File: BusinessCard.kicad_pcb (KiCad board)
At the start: 2 copper layers, 85.6 x 54 mm, 29 parts, among them U1 NT3H2111W0FHKH

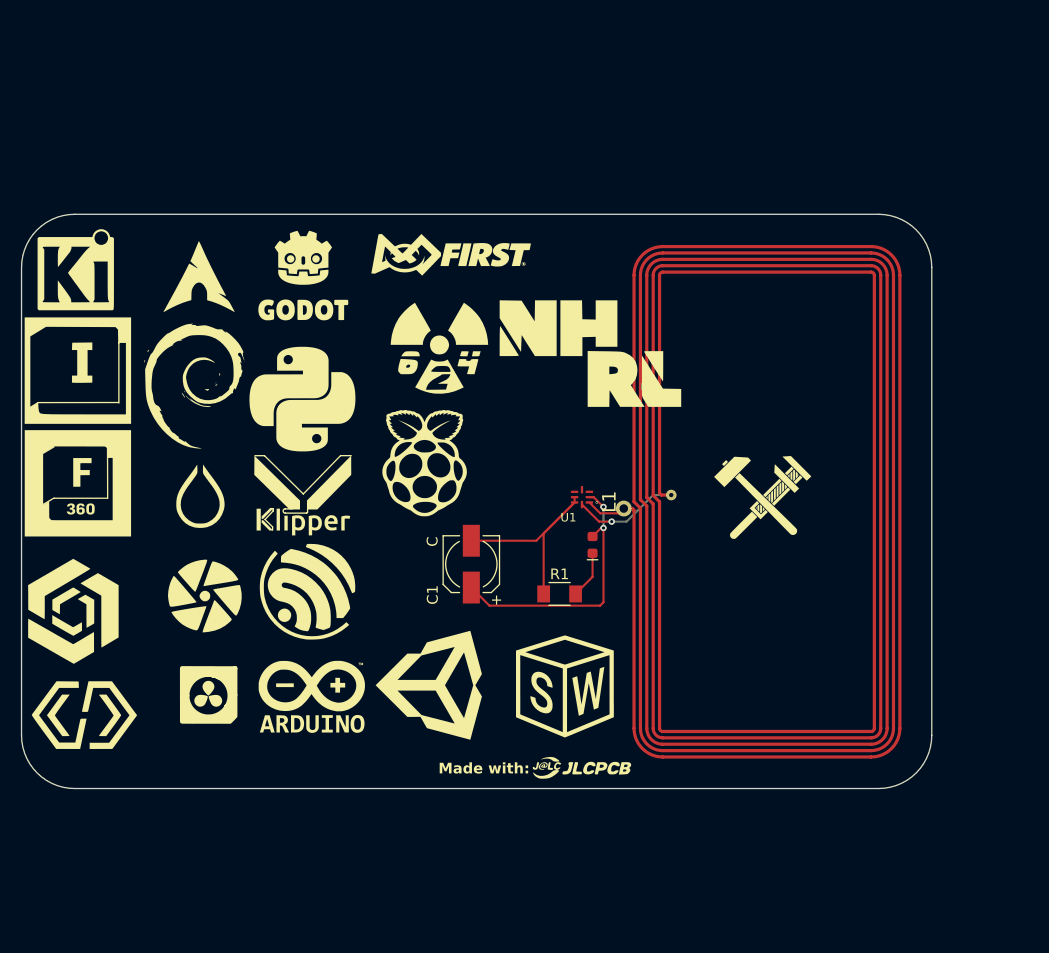
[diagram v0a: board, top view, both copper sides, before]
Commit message: Made a few design changes, started the intro
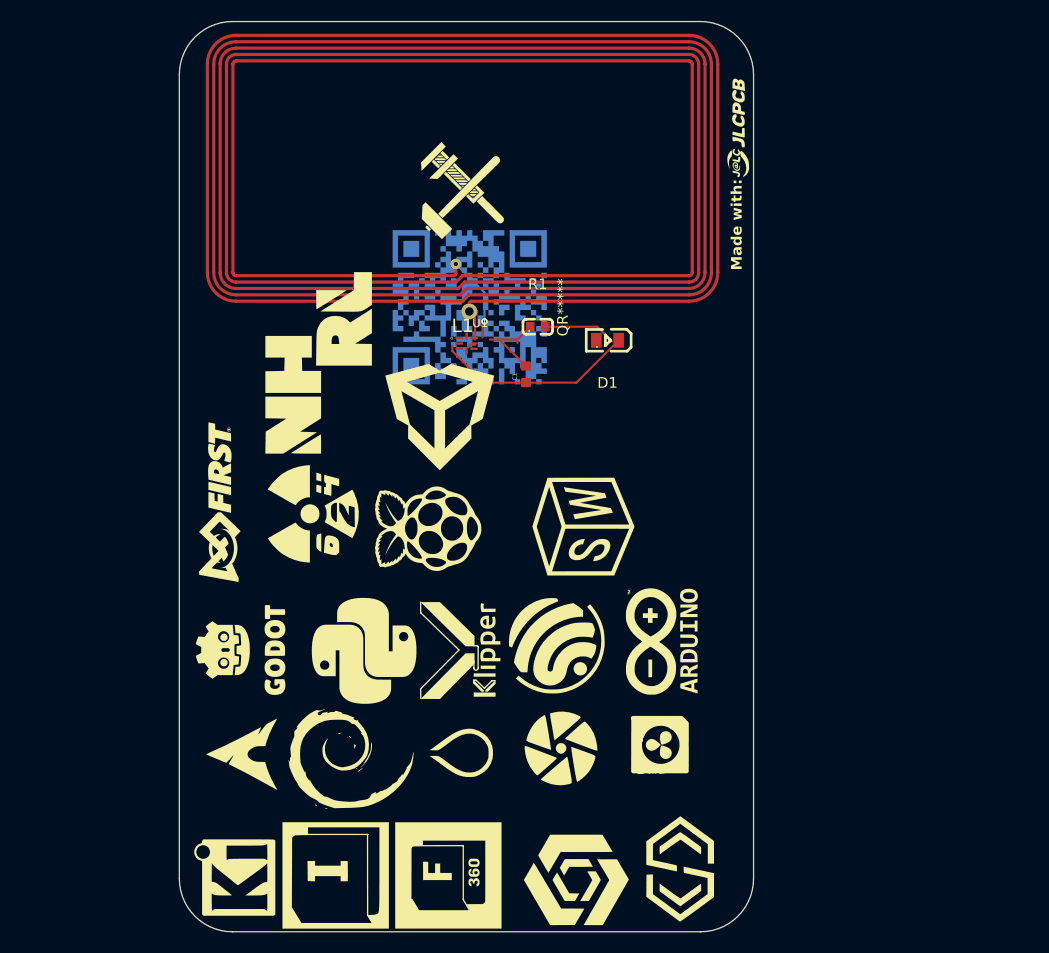
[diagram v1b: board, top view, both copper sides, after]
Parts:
- added QR*****: https://github.com/JudasLilith, nfc:https___github.com_JudasLilith, B.Cu at (116.0, 74.8)
- C1: footprint PCM_4ms_Capacitor:CP_Elec_5x5.3 -> nfc:CAPC1608X90N
- D1: footprint PCM_SparkFun-LED:LED_0603_1608Metric -> nfc:LED0805-R-RD
- R1: footprint PCM_fab:R_1206 -> nfc:C0603
- moved G*** 62.0 mm to (141.3, 57.9), turned to 90 degrees
- moved G*** 59.0 mm to (94.0, 128.4), turned to 90 degrees
- moved G*** 57.8 mm to (135.7, 127.6), turned to 90 degrees
- moved G*** 53.5 mm to (126.1, 128.5), turned to 90 degrees
- moved G*** 53.3 mm to (103.4, 128.2), turned to 90 degrees
- moved G*** 50.7 mm to (114.0, 128.2), turned to 90 degrees
- moved G*** 44.3 mm to (95.4, 116.8), turned to 90 degrees
- moved L1 42.5 mm to (115.4, 61.7), turned to 180 degrees
- moved G*** 40.4 mm to (115.4, 63.8), turned to 90 degrees
- moved G*** 40.0 mm to (133.9, 113.4), turned to 90 degrees
- moved G*** 38.0 mm to (104.8, 117.2), turned to 90 degrees
- moved G*** 34.9 mm to (95.2, 107.0), turned to 90 degrees
- moved G*** 34.4 mm to (115.2, 116.7), turned to 90 degrees
- moved G*** 33.4 mm to (134.1, 106.2), turned to 90 degrees
- moved G*** 31.9 mm to (92.5, 93.1), turned to 90 degrees
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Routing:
- net Net-(C1--): track 21.5 -> 7.87 mm
- net Net-(C1-+): track 25.3 -> 19.7 mm, vias 2 -> 0
- net Net-(D1-K): track 4.49 -> 6.88 mm
- net Net-(U1-LB): track 10.1 -> 8.21 mm
- net Net-(U1-LA): track 3.66 -> 3.05 mm
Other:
- board size 85.6 x 54 mm -> 54 x 85.6 mm
- board text added: "+1(346)-287-4367"
- board text added: "-Beginner GameDev & WebDev"
- board text added: "-FRC,NTHS,TSA & Hack Club"
- board text added: "-Hobby CAD student"
- board text added: "-Hobby Mill and CNC machinist"
- board text added: "-PCB designer"
- board text added: "-Supreme™ Archlinux user"
- board text added: "He/him"
- board text added: "Judaslilith.com"
- board text added: "Slack ID: @JudasLilith"
- board text added: "judas1lilith@gmail.com"
- board text removed: "JudasLilith"

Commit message: Final push after ordering
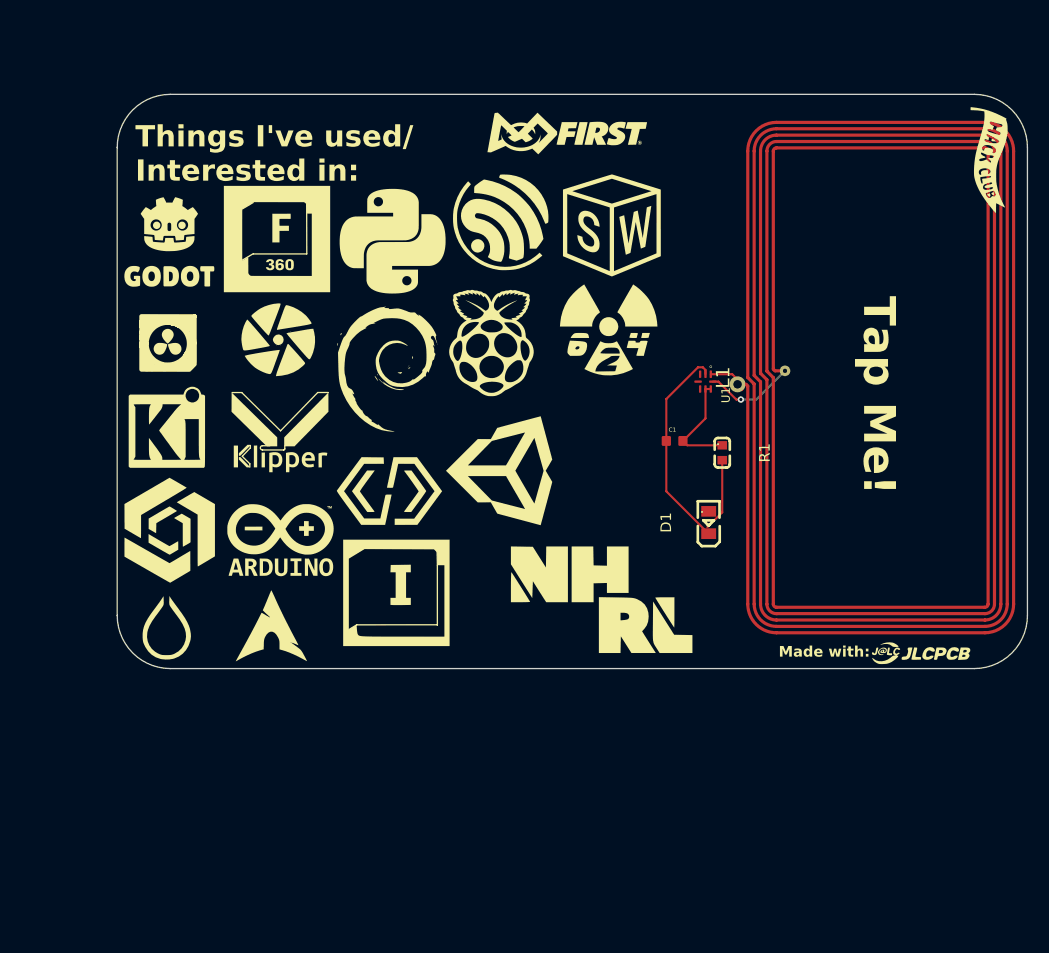
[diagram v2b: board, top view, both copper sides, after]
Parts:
- removed the G*** at (115.4, 63.8)
- removed the G*** at (116.0, 91.3)
- removed the QR***** at (116.0, 74.8)
- added G***: LOGO, nfcactual:hackClub, F.Cu at (164.9, 60.9)
- added G***: LOGO, nfcactual:moon, B.Cu at (125.9, 82.4)
- added QR*****: https://github.com/JudasLilith, nfcactual:https___github.com_JudasLilith, B.Cu at (142.2, 82.5)
- moved G*** 62.0 mm to (97.9, 68.3), turned to 0 degrees
- moved G*** 56.2 mm to (90.2, 78.1), turned to 0 degrees
- moved G*** 52.3 mm to (158.5, 107.3), turned to 0 degrees
- moved G*** 50.3 mm to (88.0, 95.8), turned to 0 degrees
- moved G*** 47.6 mm to (125.2, 58.4), turned to 0 degrees
- moved G*** 44.9 mm to (108.5, 91.9), turned to 0 degrees
- moved L1 44.0 mm to (154.7, 81.4), turned to 90 degrees
- moved G*** 42.7 mm to (87.6, 86.1), turned to 0 degrees
- moved G*** 40.2 mm to (119.0, 66.8), turned to 0 degrees
- moved G*** 38.7 mm to (108.8, 68.5), turned to 0 degrees
- moved G*** 38.4 mm to (87.8, 69.3), turned to 0 degrees
- moved G*** 37.1 mm to (98.3, 96.7), turned to 0 degrees
- moved G*** 36.8 mm to (108.3, 80.5), turned to 0 degrees
- moved G*** 34.7 mm to (128.5, 102.2), turned to 0 degrees
- moved G*** 32.7 mm to (129.1, 76.9), turned to 0 degrees
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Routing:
- net Net-(C1--): track 7.87 -> 10.1 mm
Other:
- board size 54 x 85.6 mm -> 85.6 x 54 mm
- board text added: "& more"
- board text added: "-CAD student/PCB designerr"
- board text added: "FRC,NTHS,"
- board text added: "TSA, Hack Clubr r"
- board text added: "Tap Me!"
- board text added: "Things I've used/ Interested in:"
- board text removed: "-FRC,NTHS,TSA & Hack Club"
- board text removed: "-Hobby CAD student"
- board text removed: "-PCB designer"
